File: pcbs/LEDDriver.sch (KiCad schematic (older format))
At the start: 1 part, among them J1 Conn_02x32_Counter_Clockwise

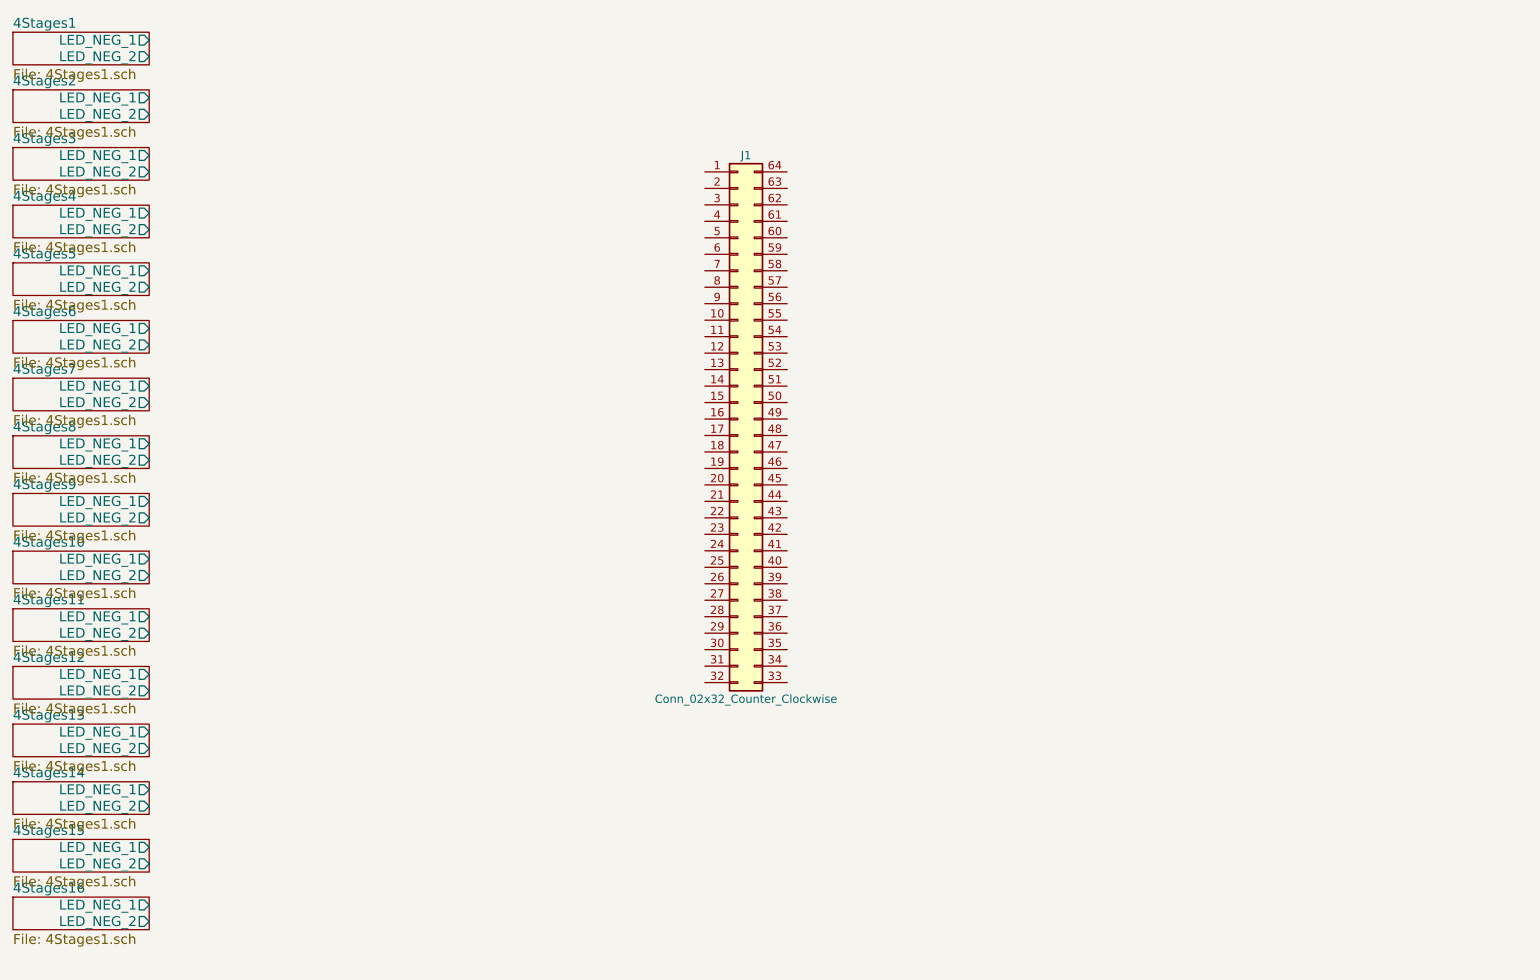
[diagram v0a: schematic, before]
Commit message: LED driver part done.
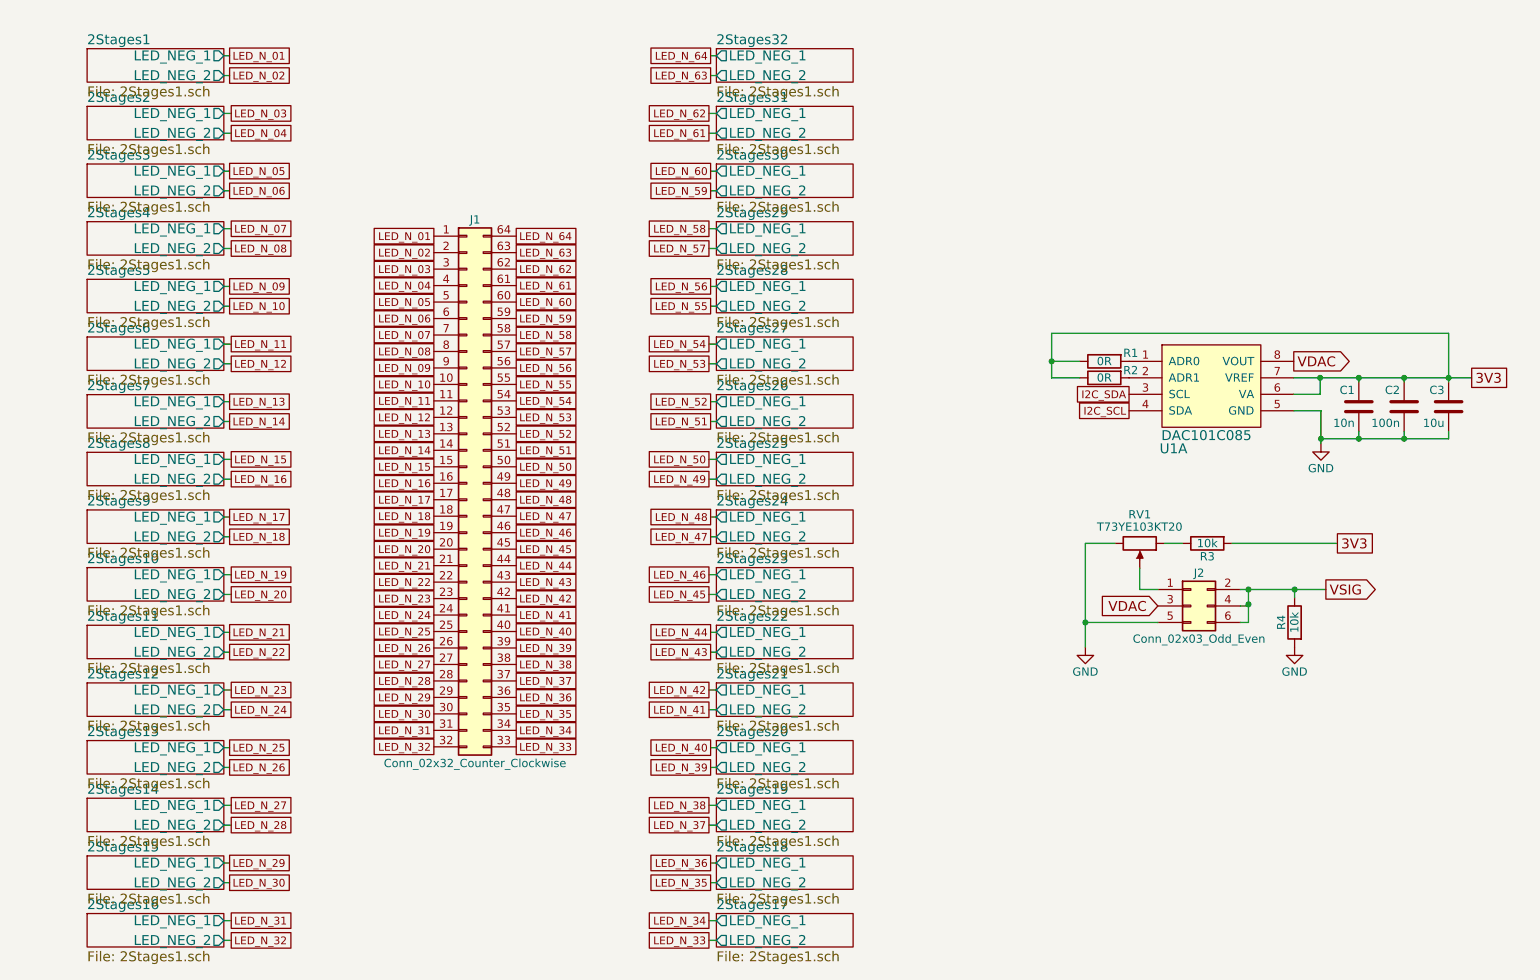
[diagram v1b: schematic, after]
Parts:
- added C1: 10n, Resistors_SMD:R_0603, symbol C
- added C2: 100n, Resistors_SMD:R_0603, symbol C
- added C3: 10u, Resistors_SMD:R_0603, symbol C
- added J2: Conn_02x03_Odd_Even, Pin_Headers:Pin_Header_Straight_2x03_Pitch2.54mm, symbol Conn_02x03_Odd_Even
- added R1, R2: 0R, Resistors_SMD:R_0603, symbol R
- added R3, R4: 10k, Resistors_SMD:R_0603, symbol R
- added RV1: T73YE103KT20, Potis:Vishay_T73YE103KT20, symbol POT
- added U1: DAC101C085, SSOP:VSSOP-8_3.0x3.0mm_Pitch0.65mm, symbol DAC101C085
- J1: footprint (none) -> Pin_Headers:Pin_Header_Straight_2x32_Pitch2.54mm; Samtec (none) -> TSW-132-07-G-D
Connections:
- net LED_N_01: now reaches J1.1 (Pin_1)
- net LED_N_10: now reaches J1.10 (Pin_10)
- net LED_N_11: now reaches J1.11 (Pin_11)
- net LED_N_12: now reaches J1.12 (Pin_12)
- net LED_N_13: now reaches J1.13 (Pin_13)
- net LED_N_14: now reaches J1.14 (Pin_14)
- net LED_N_15: now reaches J1.15 (Pin_15)
- net LED_N_16: now reaches J1.16 (Pin_16)
- net LED_N_17: now reaches J1.17 (Pin_17)
- net LED_N_18: now reaches J1.18 (Pin_18)
- net LED_N_19: now reaches J1.19 (Pin_19)
- net LED_N_02: now reaches J1.2 (Pin_2)
- net LED_N_20: now reaches J1.20 (Pin_20)
- net LED_N_21: now reaches J1.21 (Pin_21)
- net LED_N_22: now reaches J1.22 (Pin_22)
- net LED_N_23: now reaches J1.23 (Pin_23)
- net LED_N_24: now reaches J1.24 (Pin_24)
- net LED_N_25: now reaches J1.25 (Pin_25)
- net LED_N_26: now reaches J1.26 (Pin_26)
- net LED_N_27: now reaches J1.27 (Pin_27)
- net LED_N_28: now reaches J1.28 (Pin_28)
- net LED_N_29: now reaches J1.29 (Pin_29)
- net LED_N_03: now reaches J1.3 (Pin_3)
- net LED_N_30: now reaches J1.30 (Pin_30)
- net LED_N_31: now reaches J1.31 (Pin_31)
- net LED_N_32: now reaches J1.32 (Pin_32)
- net LED_N_33: now reaches J1.33 (Pin_33)
- net LED_N_34: now reaches J1.34 (Pin_34)
- net LED_N_35: now reaches J1.35 (Pin_35)
- net LED_N_36: now reaches J1.36 (Pin_36)
- net LED_N_37: now reaches J1.37 (Pin_37)
- net LED_N_38: now reaches J1.38 (Pin_38)
- net LED_N_39: now reaches J1.39 (Pin_39)
- net LED_N_04: now reaches J1.4 (Pin_4)
- net LED_N_40: now reaches J1.40 (Pin_40)
- net LED_N_41: now reaches J1.41 (Pin_41)
- net LED_N_42: now reaches J1.42 (Pin_42)
- net LED_N_43: now reaches J1.43 (Pin_43)
- net LED_N_44: now reaches J1.44 (Pin_44)
- net LED_N_45: now reaches J1.45 (Pin_45)
- net LED_N_46: now reaches J1.46 (Pin_46)
- net LED_N_47: now reaches J1.47 (Pin_47)
- net LED_N_48: now reaches J1.48 (Pin_48)
- net LED_N_49: now reaches J1.49 (Pin_49)
- net LED_N_05: now reaches J1.5 (Pin_5)
- net LED_N_50: now reaches J1.50 (Pin_50)
- net LED_N_51: now reaches J1.51 (Pin_51)
- net LED_N_52: now reaches J1.52 (Pin_52)
- net LED_N_53: now reaches J1.53 (Pin_53)
- net LED_N_54: now reaches J1.54 (Pin_54)
- net LED_N_55: now reaches J1.55 (Pin_55)
- net LED_N_56: now reaches J1.56 (Pin_56)
- net LED_N_57: now reaches J1.57 (Pin_57)
- net LED_N_58: now reaches J1.58 (Pin_58)
- net LED_N_59: now reaches J1.59 (Pin_59)
- net LED_N_06: now reaches J1.6 (Pin_6)
- net LED_N_60: now reaches J1.60 (Pin_60)
- net LED_N_61: now reaches J1.61 (Pin_61)
- net LED_N_62: now reaches J1.62 (Pin_62)
- net LED_N_63: now reaches J1.63 (Pin_63)
- net LED_N_64: now reaches J1.64 (Pin_64)
- net LED_N_07: now reaches J1.7 (Pin_7)
- net LED_N_08: now reaches J1.8 (Pin_8)
- net LED_N_09: now reaches J1.9 (Pin_9)
- new net: R1.2, U1.1 (ADR0)
- new net: R2.2, U1.2 (ADR1)
- new net: R3.1, RV1.1
- new net: J2.1 (Pin_1), RV1.2
- new net 3V3: C1.1, C2.1, C3.1, R1.1, R2.1, R3.2, U1.6 (VA), U1.7 (VREF)
- new net GND: C1.2, C2.2, C3.2, J2.5 (Pin_5), R4.2, RV1.3, U1.5 (GND)
- new net I2C_SCL: U1.4 (SDA)
- new net I2C_SDA: U1.3 (SCL)
- new net VDAC: J2.3 (Pin_3), U1.8 (VOUT)
- new net VSIG: J2.2 (Pin_2), J2.4 (Pin_4), J2.6 (Pin_6), R4.1
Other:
- moved on the sheet: J1
